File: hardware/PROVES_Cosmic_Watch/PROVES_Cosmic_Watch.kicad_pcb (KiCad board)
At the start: 4 copper layers, 88 x 95 mm, 45 parts, among them J1 USB_B_Micro, J2 DF11, J3 Conn_Coaxial, U2 LT3461ES6-TRPBF, U3 LT1807, U4 MICROFC-60035-SMT-TR

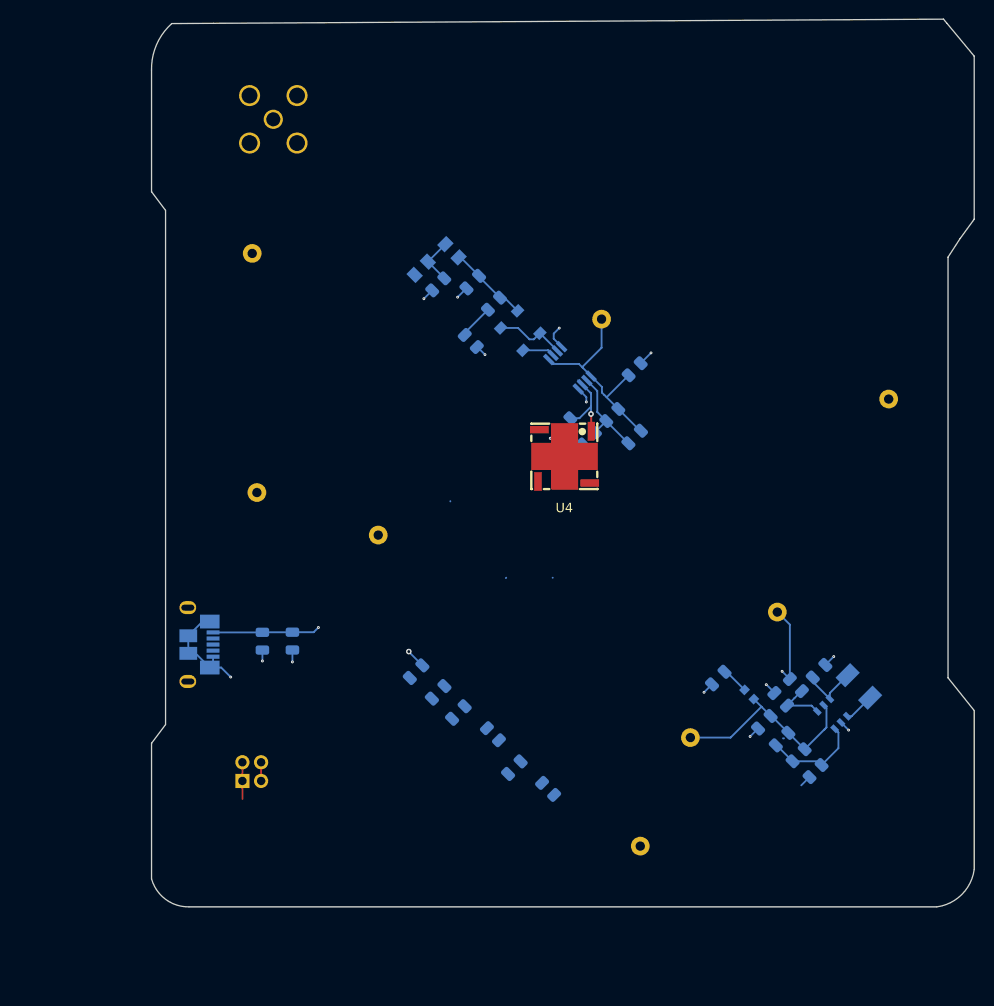
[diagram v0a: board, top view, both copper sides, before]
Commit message: Layout Updates
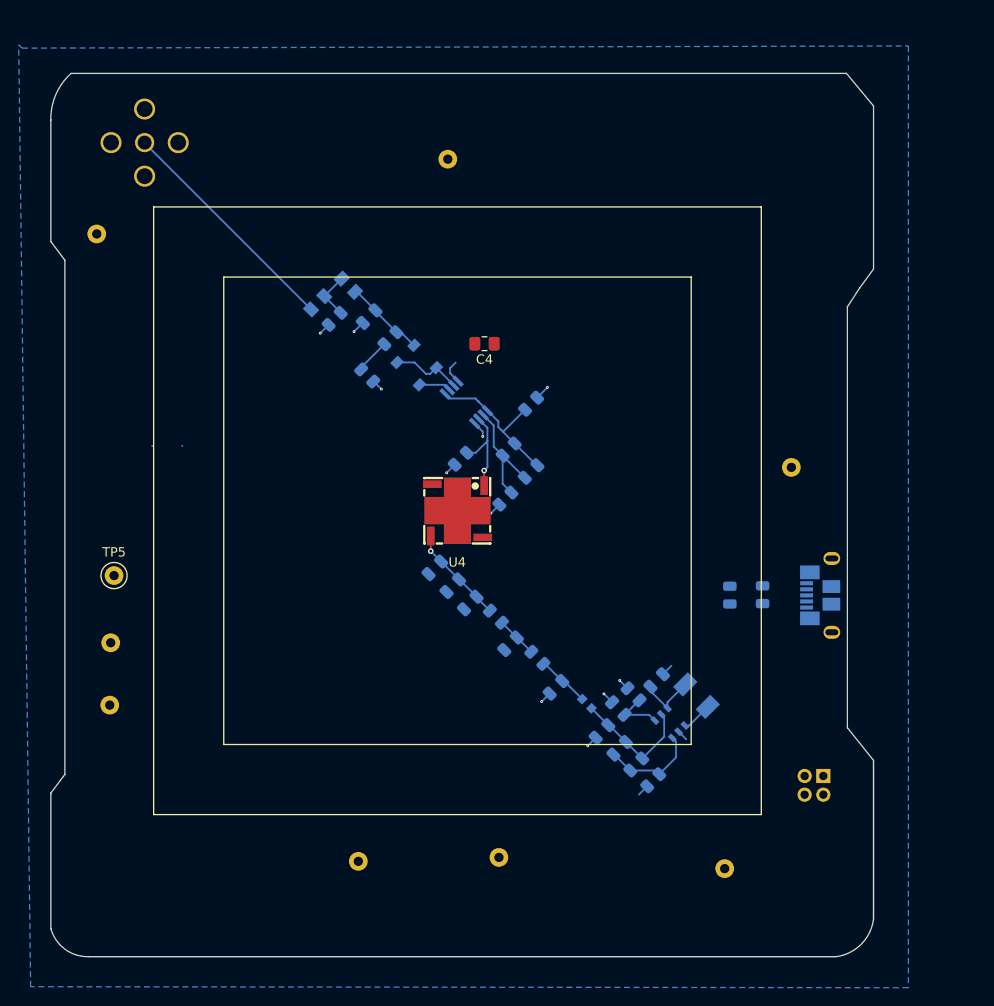
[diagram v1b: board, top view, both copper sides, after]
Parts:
- added C4: 10uF, Capacitor_SMD:C_0805_2012Metric_Pad1.18x1.45mm_HandSolder, F.Cu at (135.7, 81.2)
- added TP5: Bias Voltage, TestPoint:TestPoint_Keystone_5000-5004_Miniature, F.Cu at (96.1, 106.0)
- TP3: value GND -> GND Test Point
- TP6: value 5V -> 5V Test Point
- TP7: value V+ Bias -> FB Test Point
- TP8: value V+ Out -> Output Voltage Test Point
- TP9: value SHDN -> SHDN Test Point
- moved J1 66.4 mm to (171.5, 108.1), turned to 180 degrees
- moved J2 60.2 mm to (171.0, 128.4), turned to 0 degrees
- moved C14 53.7 mm to (165.5, 108.0), turned to 90 degrees
- moved C15 47.0 mm to (162.0, 108.1), turned to 90 degrees
- moved TP6 34.0 mm to (95.6, 119.8)
- moved TP7 30.2 mm to (122.2, 136.6)
- moved TP9 28.0 mm to (161.4, 137.3), turned to 0 degrees
- moved TP8 24.2 mm to (137.3, 136.1)
- moved TP1 23.7 mm to (131.8, 61.4)
- moved TP3 22.4 mm to (95.7, 113.2)
- moved L1 17.4 mm to (158.4, 118.8)
- moved L2 17.4 mm to (146.7, 119.7)
- moved C16 17.4 mm to (150.0, 120.2)
- moved C5 17.4 mm to (154.1, 117.2)
- moved C6 17.4 mm to (150.2, 124.5)
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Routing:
- net +5V: track 35.5 -> 10.2 mm, vias 3 -> 1
- net Post Processed Signal: track 0.00 -> 25.2 mm
- net GND: track 35.2 -> 17.1 mm, vias 15 -> 10
- net V_Out: track 22.5 -> 13.5 mm
- net Net-(U4-CATHODE): track 2.14 -> 10.6 mm
- net Net-(U3B-+): track 23.1 -> 17.1 mm
- net Net-(C10-Pad1): track 0.00 -> 4.44 mm
- net V_Bias: track 2.94 -> 5.72 mm
- net Net-(U3A--): track 10.7 -> 13.4 mm
- net SiPM Signal: track 8.75 -> 11.0 mm
- added copper zone on B.Cu, net +5V
- added copper zone on In1.Cu, net GND
- removed copper zone on In1.Cu, net +5V
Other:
- board size 88 x 95 mm -> 88 x 94.5 mm
